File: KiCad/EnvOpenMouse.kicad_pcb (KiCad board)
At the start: 2 copper layers, 34 x 107.5 mm, 74 parts, among them J1 Button, J10 0.8mm BM03B, J11 Conn_02x02_Top_Bottom, J12 0.8mm BM03B, J13 0.8mm BM03B, J14 0.8mm BM03B, J15 0.8mm BM03B, J16 Conn_01x14, J2 Conn_01x03, J3 Button, J4 Conn_02x02_Top_Bottom, J5 Conn_02x02_Top_Bottom, J6 Conn_02x02_Top_Bottom, J7 Conn_02x02_Top_Bottom, J8 Conn_02x02_Top_Bottom, J9 0.8mm BM03B, SW1 SW_Push_SPDT, SW2 SW_Push_SPDT, SW3 SW_Push_SPDT, SW4 SW_Push_SPDT, SW5 SW_Push_SPDT, SW6 SW_Push_SPDT, SW7 SW_Push_SPDT, SW8 SW_Push_SPDT, SW9 SW_Push_SPDT, U1 AP2112K-3.3, U2 TLV70218DBVR, U3 RP2040, U4 PMW3360DM-T2QU, Y1 3225_4P 12MHz

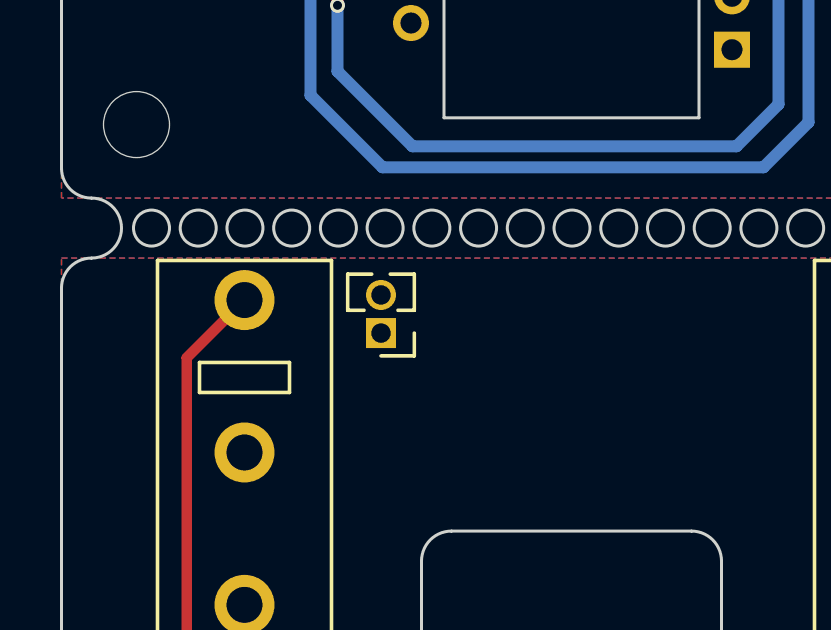
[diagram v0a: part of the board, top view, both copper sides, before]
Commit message: generated production files
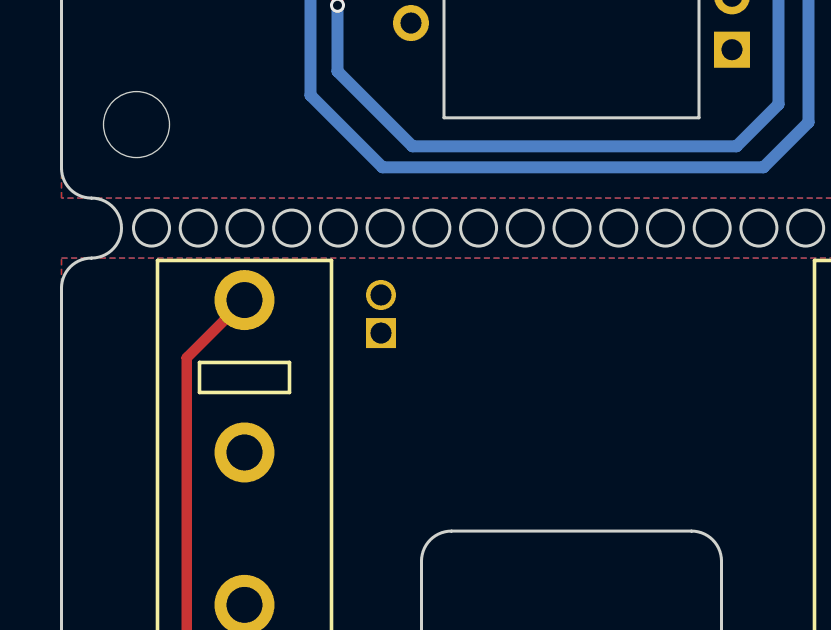
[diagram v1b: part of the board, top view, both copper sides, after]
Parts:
- J4: footprint Connector_PinHeader_1.27mm:PinHeader_1x02_P1.27mm_Vertical -> Connector_PinSocket_1.27mm:PinSocket_1x02_P1.27mm_Vertical; moved to B.Cu
- turned J4 to 0 degrees
